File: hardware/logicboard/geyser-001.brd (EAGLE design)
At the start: 47 x 47 mm, 13 parts, among them T1 2SC1815

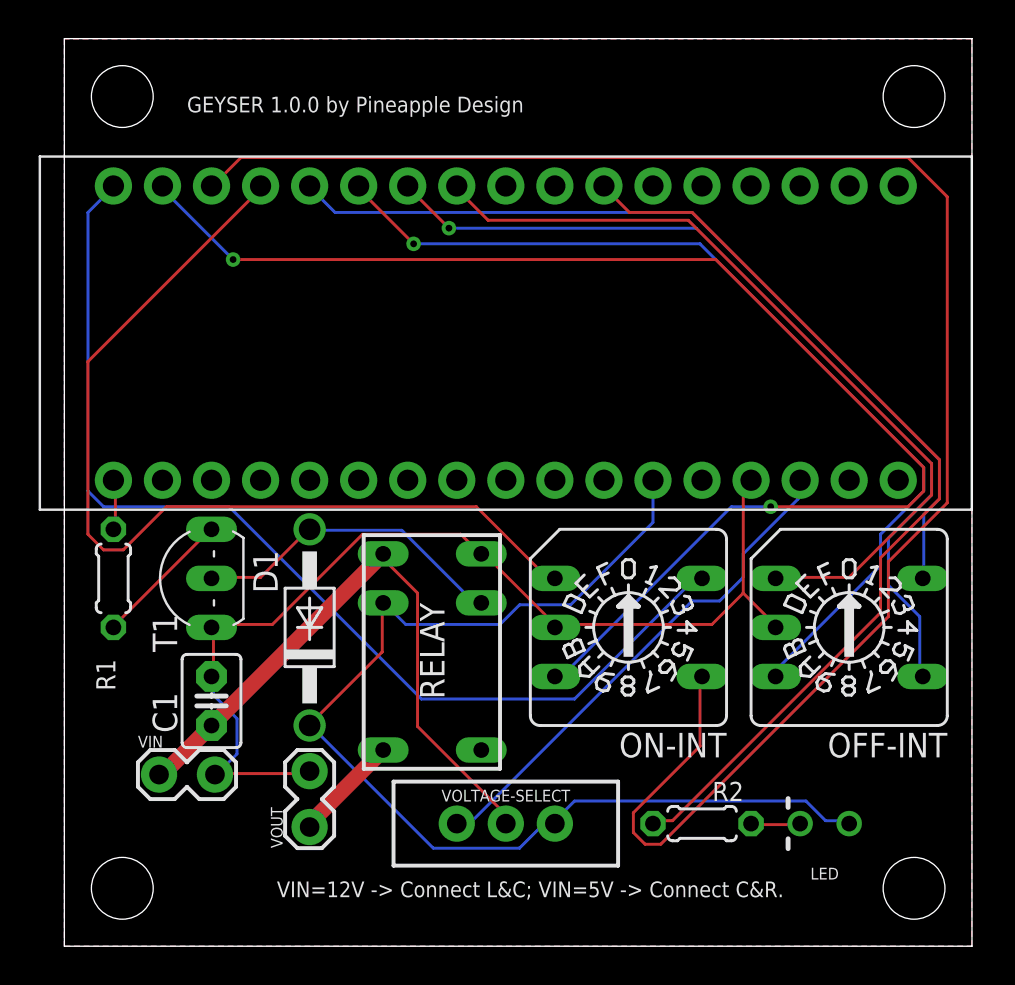
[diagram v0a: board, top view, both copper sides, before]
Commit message: New layout.
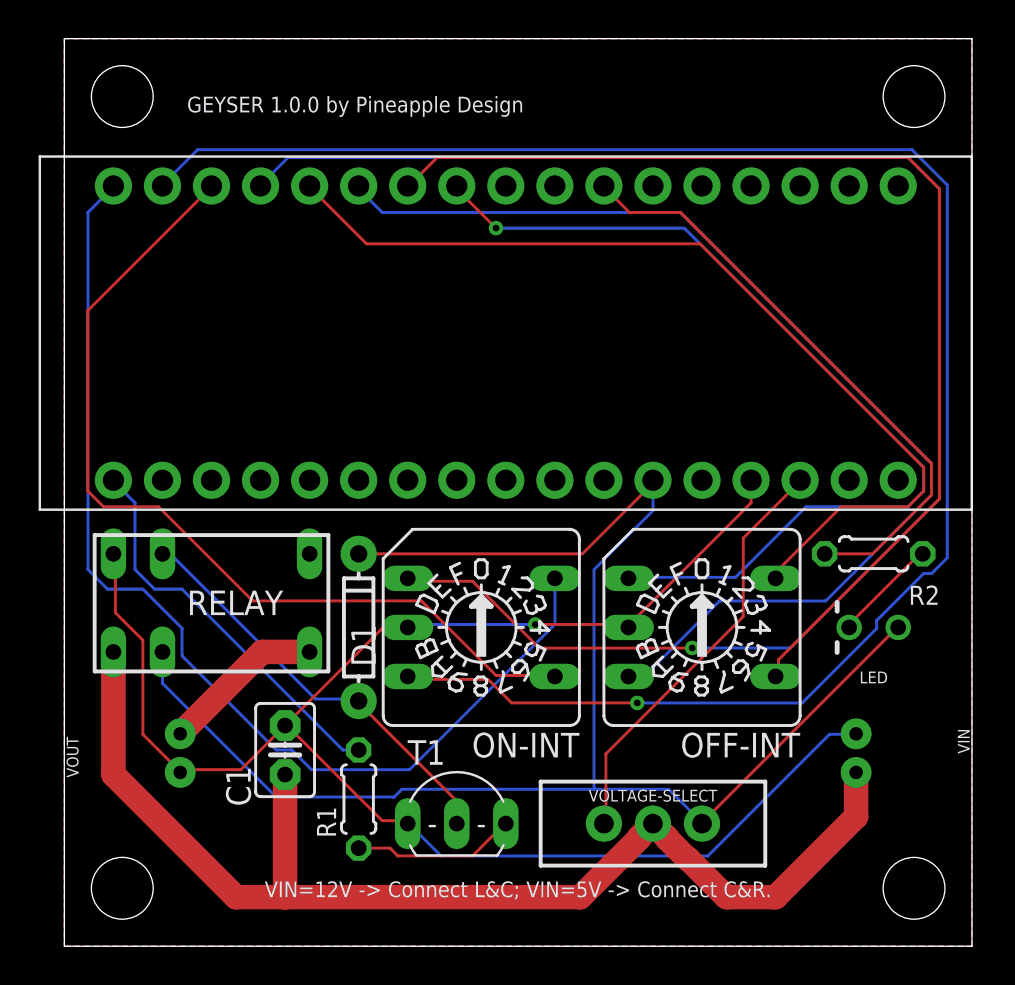
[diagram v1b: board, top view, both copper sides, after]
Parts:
- C1: value (none) -> 104
- D1: value 1N4004 -> 200mA/100V/1V; device diode:DO41-10 -> SparkFun-DiscreteSemi:DIODE-1N4148
- VIN, VOUT: device SparkFun-Connectors:1X02_LOCK -> SparkFun-Connectors:JST-2-PTH-NS
- moved VIN 35.9 mm to (41.0, 10.0), turned to 270 degrees
- moved T1 18.0 mm to (20.3, 6.35), turned to 0 degrees
- moved R1 17.1 mm to (15.2, 7.62)
- moved R2 16.6 mm to (41.9, 20.3)
- moved RELAY 11.7 mm to (7.62, 17.8), turned to 0 degrees
- moved LED 10.5 mm to (41.9, 16.5)
- moved VOUT 7.63 mm to (6.00, 10.0)
- moved ON-INT 7.62 mm to (21.6, 16.5)
- moved VOLTAGE-SELECT 7.62 mm to (30.5, 6.35)
- moved OFF-INT 7.62 mm to (33.0, 16.5)
- moved C1 4.58 mm to (11.4, 10.2)
- moved D1 2.54 mm to (15.2, 16.5)
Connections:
- removed net N$1: RELAY.5, VOUT.1
- new net VOUT: RELAY.5, VOUT.2
- net GND: now also VIN.1, VOUT.1; no longer VIN.2, VOUT.2
- net VDD: now also VIN.2; no longer VIN.1
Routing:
- net N$9: track 90.4 -> 46.6 mm
- net N$10: track 48.7 -> 84.8 mm, vias 0 -> 1
- net GND: track 54.5 -> 84.5 mm, vias 0 -> 1
- net VDD: track 32.9 -> 61.0 mm
- net N$8: track 69.9 -> 93.4 mm, vias 2 -> 1
- net VCC: track 59.0 -> 81.5 mm
- net RELAYDRIVE: track 2.60 -> 20.5 mm
- net LEDDRIVE: track 48.8 -> 31.4 mm
- net N$6: track 45.8 -> 57.6 mm, vias 1 -> 0
- net VOUT: track 0.00 -> 8.46 mm
- net N$5: track 49.4 -> 56.9 mm, vias 1 -> 0
- net N$11: track 42.1 -> 48.7 mm, vias 0 -> 1
- net N$1: track 5.57 -> 0.00 mm
- net N$4: track 16.6 -> 21.8 mm
- net VIN: track 26.4 -> 22.0 mm
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- added copper zone on layer 1, net N$1
- added copper zone on layer 16, net N$12
- removed copper zone on layer 1, net N$12
- removed copper zone on layer 16, net N$13
